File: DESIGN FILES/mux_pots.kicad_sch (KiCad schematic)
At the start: 19 parts, among them U701 CD74HC4067

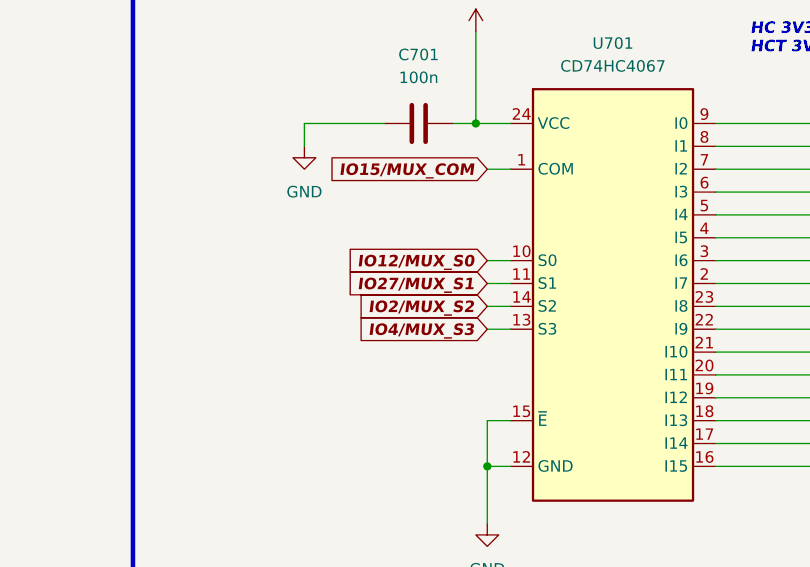
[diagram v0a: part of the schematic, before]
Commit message: updates
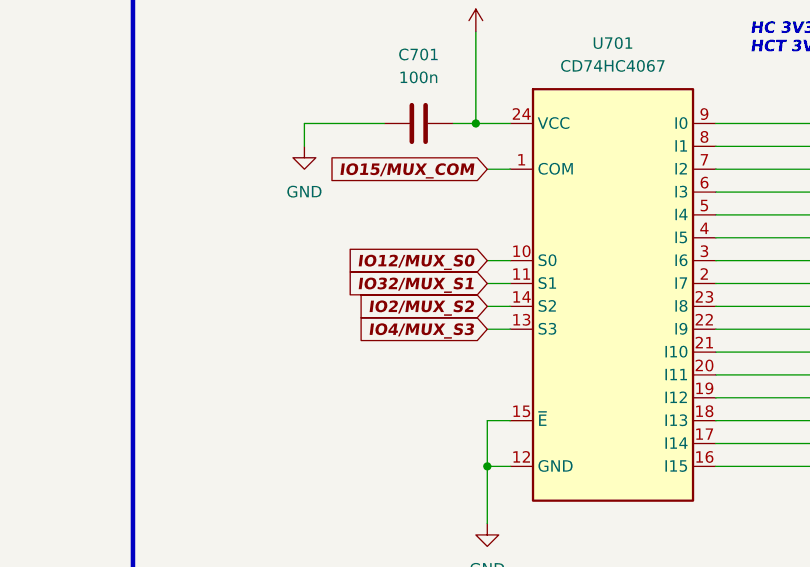
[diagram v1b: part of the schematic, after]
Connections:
- net IO27/MUX_S1 renamed IO32/MUX_S1
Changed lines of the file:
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@@
+    )
+  )
+  (global_label "IO32{slash}MUX_S1" (shape input) (at 306.07 139.7 180) (fields_autoplaced)
+    (effects (font (size 1.27 1.27) (thickness 0.254) bold italic) (justify right))
+    (property "Intersheet References" "${INTERSHEET_REFS}" (id 0) (at 290.1481 139.827 0)
+      (effects (font (size 1.27 1.27) (thickness 0.254) bold italic) (justify right) hide)
     )
   )
@@
     )
   )
-  (global_label "IO27{slash}MUX_S1" (shape input) (at 306.07 139.7 180) (fields_autoplaced)
-    (effects (font (size 1.27 1.27) (thickness 0.254) bold italic) (justify right))
-    (property "Intersheet References" "${INTERSHEET_REFS}" (id 0) (at 290.1481 139.827 0)
-      (effects (font (size 1.27 1.27) (thickness 0.254) bold italic) (justify right) hide)
-    )
-  )
